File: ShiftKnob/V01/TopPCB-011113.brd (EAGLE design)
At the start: 33 x 33 mm, 8 parts

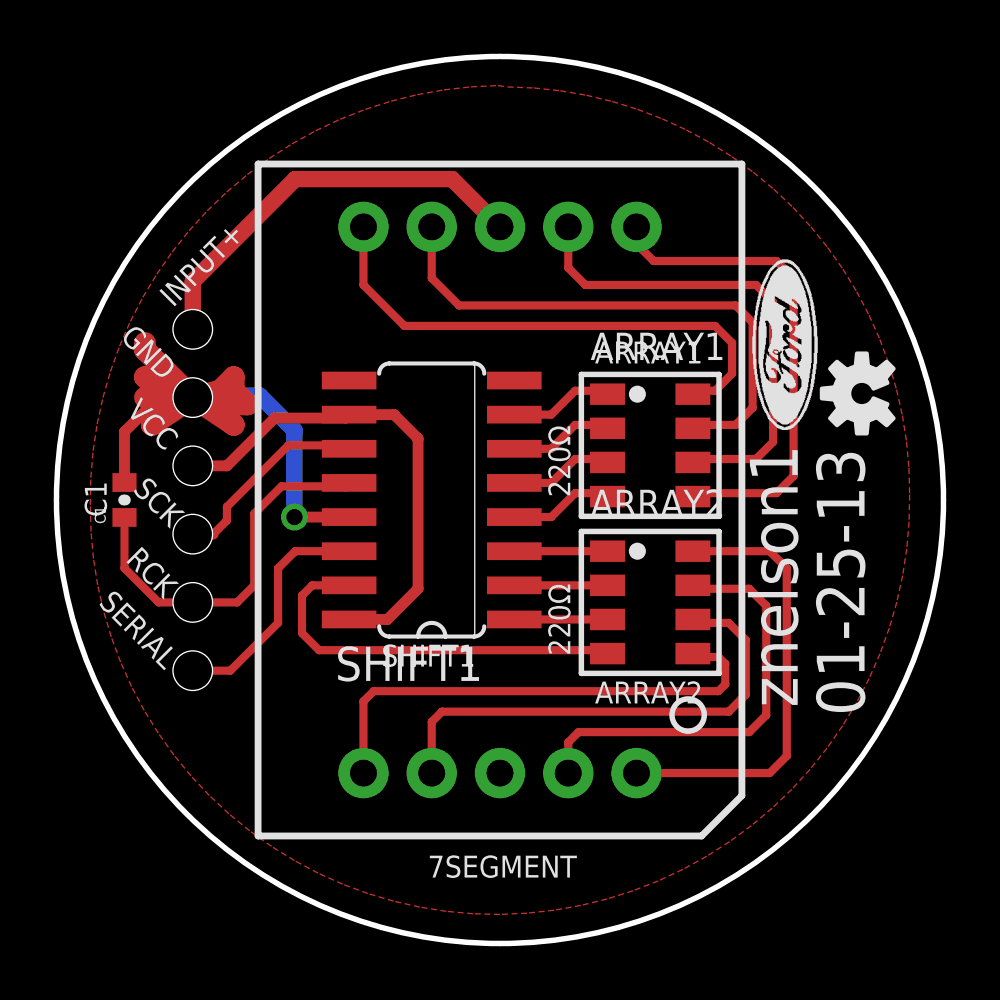
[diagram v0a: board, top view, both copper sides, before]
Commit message: adjust silk screen for vector font.
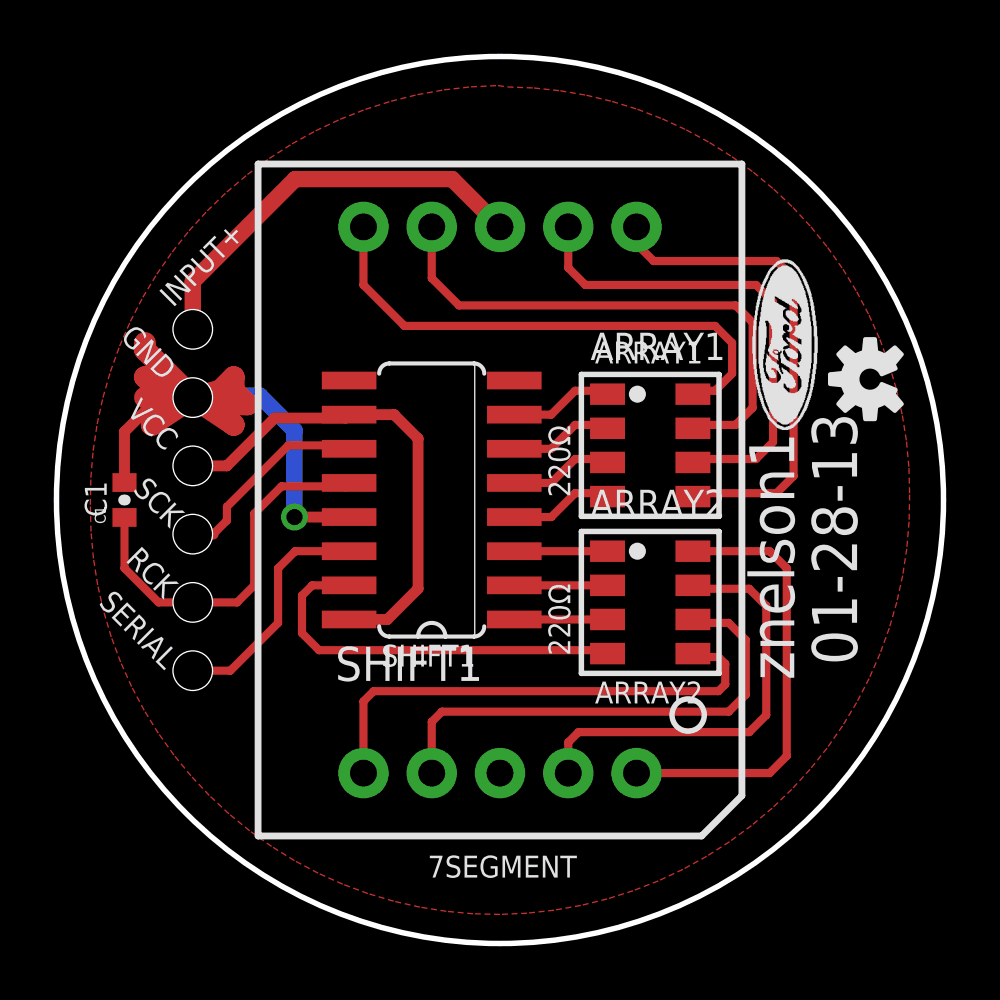
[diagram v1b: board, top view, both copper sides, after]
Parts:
- moved U$2 5.60 mm to (25.7, 22.9)
- moved U$1 0.61 mm to (31.5, 22.3)
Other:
- board text added: "01-28-13"
- board text removed: "01-25-13"
